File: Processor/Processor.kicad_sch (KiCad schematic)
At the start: 25 parts, among them J1 Buss, U1 MC6800, U2 74LS74, U3 74LS00, U4 74LS245, U7 GAL22V10, U8 74LS04, Y1 2.0MHz

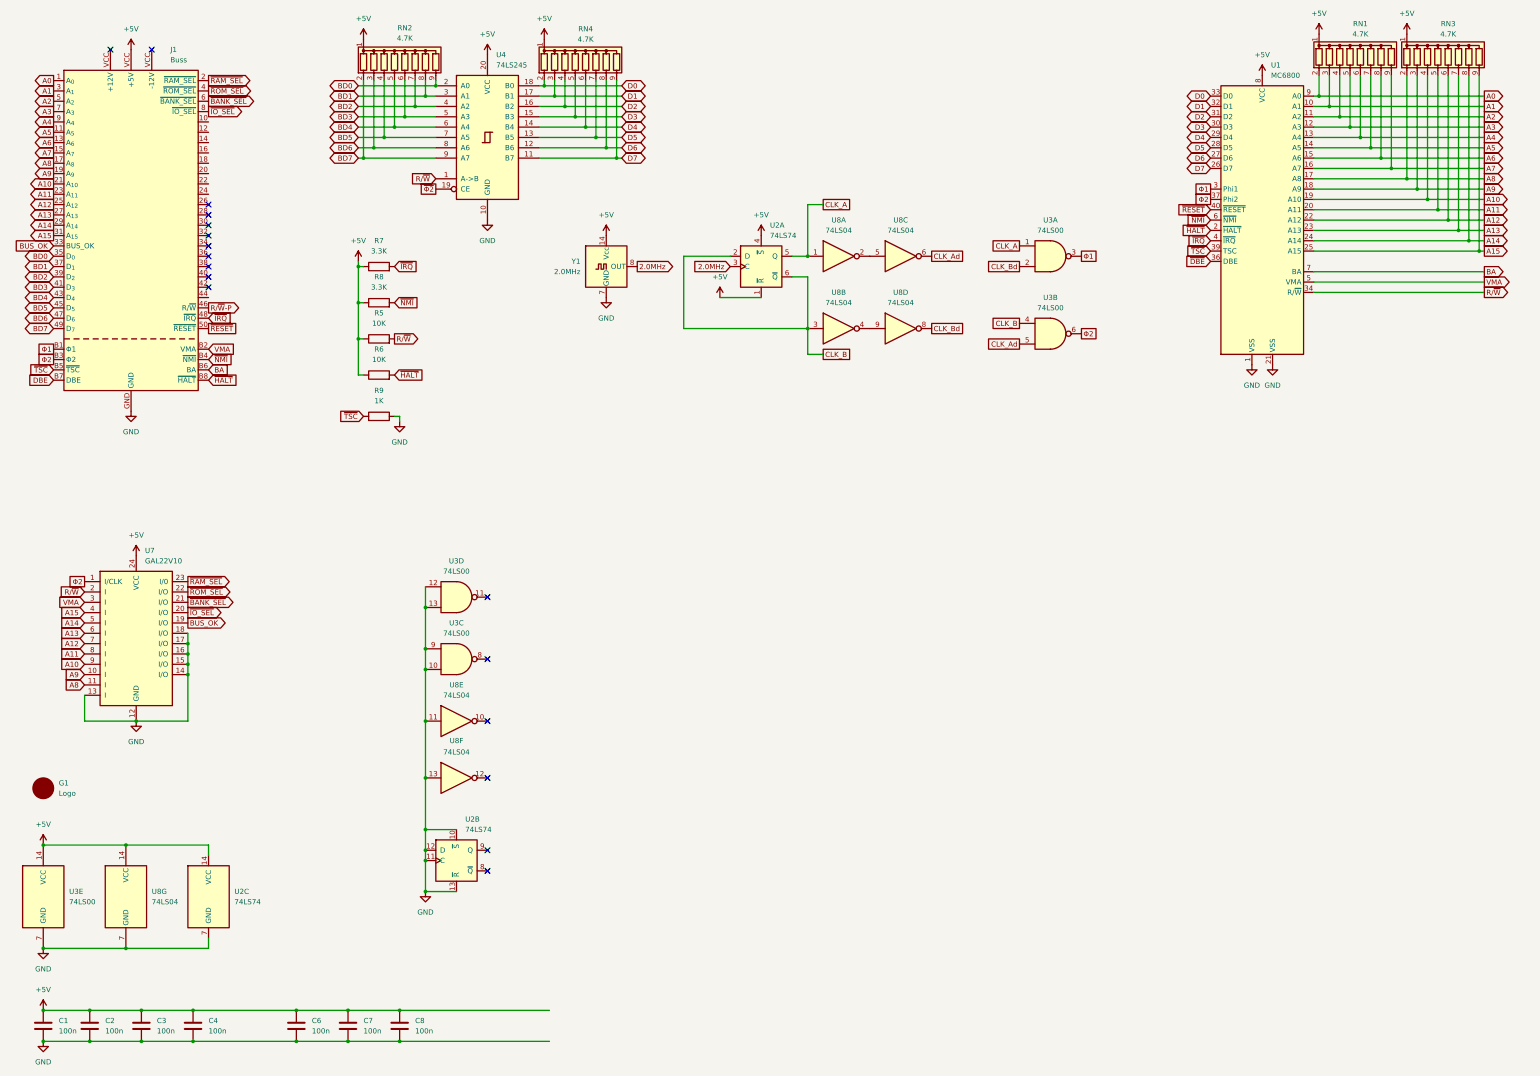
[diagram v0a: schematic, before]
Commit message: ordered v01 of the cpu
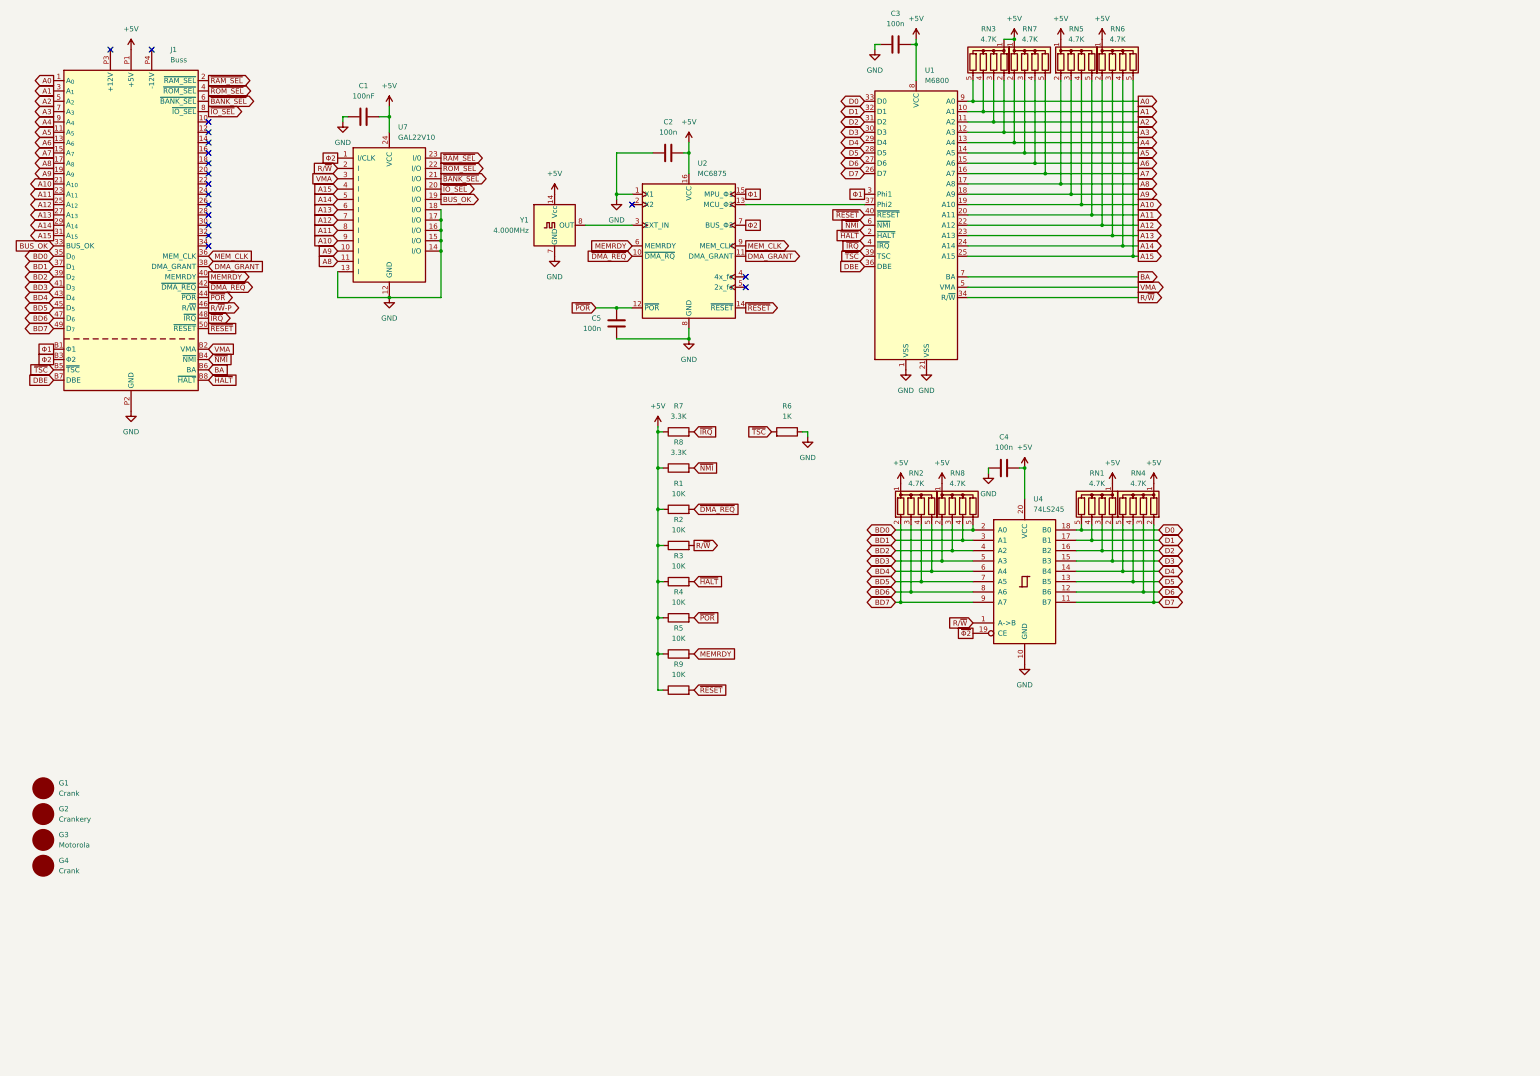
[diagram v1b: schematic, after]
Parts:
- removed C6, C7, C8: 100n, Capacitor_THT:C_Disc_D3.0mm_W1.6mm_P2.50mm, symbol Device:C
- removed R6: 10K, Resistor_THT:R_Axial_DIN0204_L3.6mm_D1.6mm_P5.08mm_Horizontal, symbol Device:R
- removed RN1, RN2, RN3, RN4: 4.7K, Resistor_THT:R_Array_SIP9, symbol Device:R_Network08
- removed U2: 74LS74, Package_DIP:DIP-14_W7.62mm, symbol 74xx:74LS74
- removed U3: 74LS00, Package_DIP:DIP-14_W7.62mm, symbol 74xx:74LS00
- removed U8: 74LS04, Package_DIP:DIP-14_W7.62mm, symbol 74xx:74LS04
- added C5: 100n, 0-Footprints:C_Disc_D5.0mm_W2.5mm_P5.00mm, symbol Device:C
- added G2: Crankery, 0-Footprints:crankery_small, symbol 0-Symbols:Logo
- added G3: Motorola, 0-Footprints:Motorola, symbol 0-Symbols:Logo
- added G4: Crank, 0-Footprints:Crank, symbol 0-Symbols:Logo
- added R1, R2, R3, R4, R9: 10K, 0-Footprints:R_Axial_DIN0204_L3.6mm_D1.6mm_P7.62mm_Horizontal, symbol Device:R
- added RN1, RN2, RN3, RN4, RN5, RN6, RN7, RN8: 4.7K, 0-Footprints:R_Array_SIP5, symbol Device:R_Network04
- added U2: MC6875, 0-Footprints:DIP-16_W7.62mm, symbol 0-Symbols:MC6875
- C1: value 100n -> 100nF; footprint Capacitor_THT:C_Disc_D3.0mm_W1.6mm_P2.50mm -> 0-Footprints:C_Disc_D5.0mm_W2.5mm_P5.00mm
- C2, C3, C4: footprint Capacitor_THT:C_Disc_D3.0mm_W1.6mm_P2.50mm -> 0-Footprints:C_Disc_D5.0mm_W2.5mm_P5.00mm
- G1: value Logo -> Crank
- R5, R7, R8: footprint Resistor_THT:R_Axial_DIN0204_L3.6mm_D1.6mm_P5.08mm_Horizontal -> 0-Footprints:R_Axial_DIN0204_L3.6mm_D1.6mm_P7.62mm_Horizontal
- R6: renamed from R9; footprint Resistor_THT:R_Axial_DIN0204_L3.6mm_D1.6mm_P5.08mm_Horizontal -> 0-Footprints:R_Axial_DIN0204_L3.6mm_D1.6mm_P7.62mm_Horizontal
- U1: value MC6800 -> M6800; footprint Package_DIP:DIP-40_W15.24mm -> 0-Footprints:DIP-40_W15.24mm
- U4: footprint Package_DIP:DIP-20_W7.62mm -> 0-Footprints:DIP-20_W7.62mm
- U7: footprint Package_DIP:DIP-24_W7.62mm -> 0-Footprints:DIP-24_W7.62mm
- Y1: value 2.0MHz -> 4.000MHz; footprint Oscillator:Oscillator_DIP-14 -> 0-Footprints:Oscillator_DIP-14
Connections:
- net ~{DBE} is gone; now on net DBE: U1.36 (DBE)
- net +5V: now also C1.2, C2.2, C3.2, C4.2, J1.P1 (+5V), R1.1, R2.1, R3.1, R4.1, R9.1, RN1.1 (common), RN2.1 (common), RN3.1 (common), RN4.1 (common), RN5.1 (common), RN6.1 (common), RN7.1 (common), RN8.1 (common), U2.16 (VCC); no longer C1.1, C2.1, C3.1, C4.1, J1.VCC (-12V)
- net A0: now also RN3.5 (R4)
- net A1: now also RN3.4 (R3)
- net A10: now also RN5.4 (R3)
- net A11: now also RN5.5 (R4)
- net A12: now also RN6.2 (R1)
- net A13: now also RN6.3 (R2)
- net A14: now also RN6.4 (R3)
- net A15: now also RN6.5 (R4)
- net A2: now also RN3.3 (R2)
- net A3: now also RN3.2 (R1)
- net A4: now also RN7.2 (R1)
- net A5: now also RN7.3 (R2)
- net A6: now also RN7.4 (R3)
- net A7: now also RN7.5 (R4)
- net A8: now also RN5.2 (R1)
- net A9: now also RN5.3 (R2)
- net BD0: now also RN8.5 (R4)
- net BD1: now also RN8.4 (R3)
- net BD2: now also RN8.3 (R2)
- net BD3: now also RN8.2 (R1)
- net BD4: now also RN2.5 (R4)
- net BD5: now also RN2.4 (R3)
- net BD6: now also RN2.3 (R2)
- net BD7: now also RN2.2 (R1)
- net D0: now also RN1.5 (R4)
- net D1: now also RN1.4 (R3)
- net D2: now also RN1.3 (R2)
- net D3: now also RN1.2 (R1)
- net D4: now also RN4.5 (R4)
- net D5: now also RN4.4 (R3)
- net D6: now also RN4.3 (R2)
- net D7: now also RN4.2 (R1)
- net GND: now also C1.1, C2.1, C3.1, C4.1, J1.P2 (GND), C5.2, U2.1 (X1), U2.8 (GND); no longer C1.2, C2.2, C3.2, C4.2, J1.GND
- net R/~{W}: now also R2.2; no longer R5.2
- net ~{HALT}: now also R3.2
- net ~{RESET}: now also R9.2, U2.14 (~{RESET})
- net Φ1: now also U2.15 (MPU_Φ1)
- net Φ2: now also U2.7 (BUS_Φ2); no longer U1.37 (Phi2)
- net MEM_CLK: now reaches J1.36 (MEM_CLK)
- net MEM_CLK: now also U2.9 (MEM_CLK)
- net DMA_GRANT: now reaches J1.38 (DMA_GRANT)
- net DMA_GRANT: now also U2.11 (DMA_GRANT)
- net MEMRDY: now reaches J1.40 (MEMRDY)
- net MEMRDY: now also R5.2, U2.6 (MEMRDY)
- net ~{DMA_REQ}: now reaches J1.42 (~{DMA_REQ})
- net ~{DMA_REQ}: now also R1.2, U2.10 (~{DMA_RQ})
- net ~{POR}: now reaches J1.44 (~{POR})
- net ~{POR}: now also C5.1, R4.2, U2.12 (~{POR})
- net 2.0MHz: no longer names the net of Y1.8 (OUT)
- net 2.0MHz: now also U2.3 (EXT_IN)
- new net: U1.37 (Phi2), U2.13 (MCU_Φ2)
- no-connect marks 17 -> 18
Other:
- moved on the sheet: C2, C3, C4, R6, R7, R8, U1, U4, U7, Y1
